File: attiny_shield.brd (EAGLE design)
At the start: 100 x 80 mm, 10 parts, among them IC1 TINY13-20PU

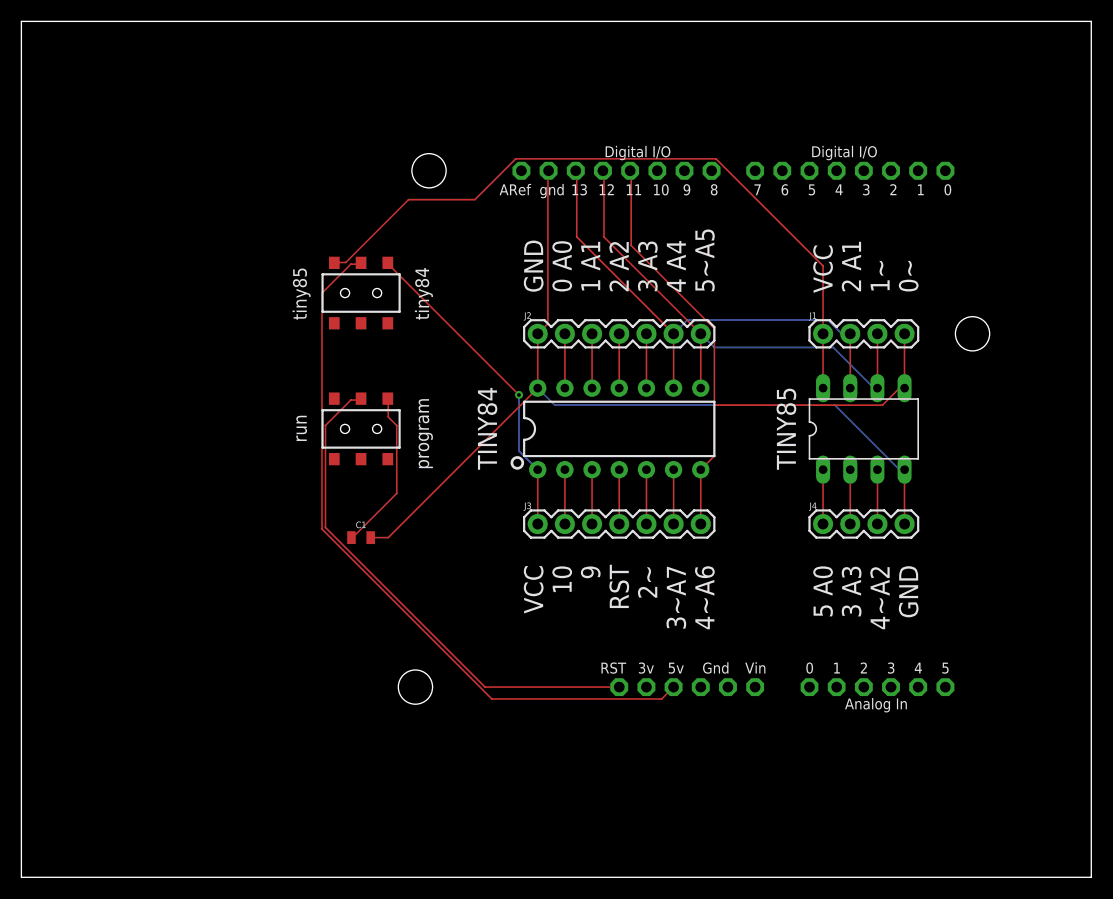
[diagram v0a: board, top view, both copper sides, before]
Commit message: named
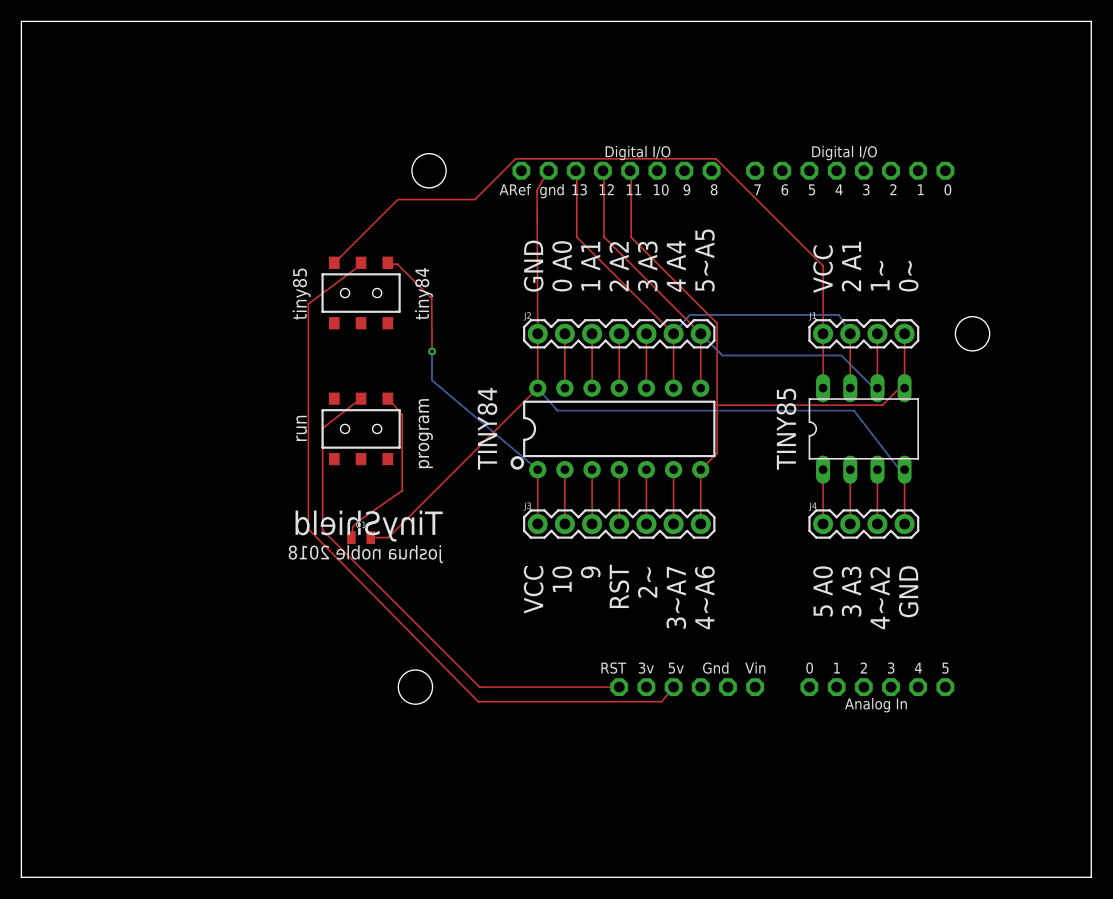
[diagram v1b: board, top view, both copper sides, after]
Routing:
- net VCC: track 66.9 -> 69.0 mm
- net N$9: track 15.1 -> 16.3 mm
- net VCC_84: track 30.2 -> 31.2 mm
- net N$1: track 46.8 -> 47.6 mm
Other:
- board text added: "TinyShield"
- board text added: "joshua noble 2018"
